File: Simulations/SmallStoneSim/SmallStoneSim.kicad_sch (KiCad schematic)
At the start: 77 parts, among them Q1 2N5088, Q2 2N5087, Q3 2N5088, Q4 2N5087, Q5 2N5087, Q6 2N5088, Q7 2N5088, SW1 SW_SPDT, SW2 SW_SPDT, U1 LM13700, U2 LM13700, U3 LM13700

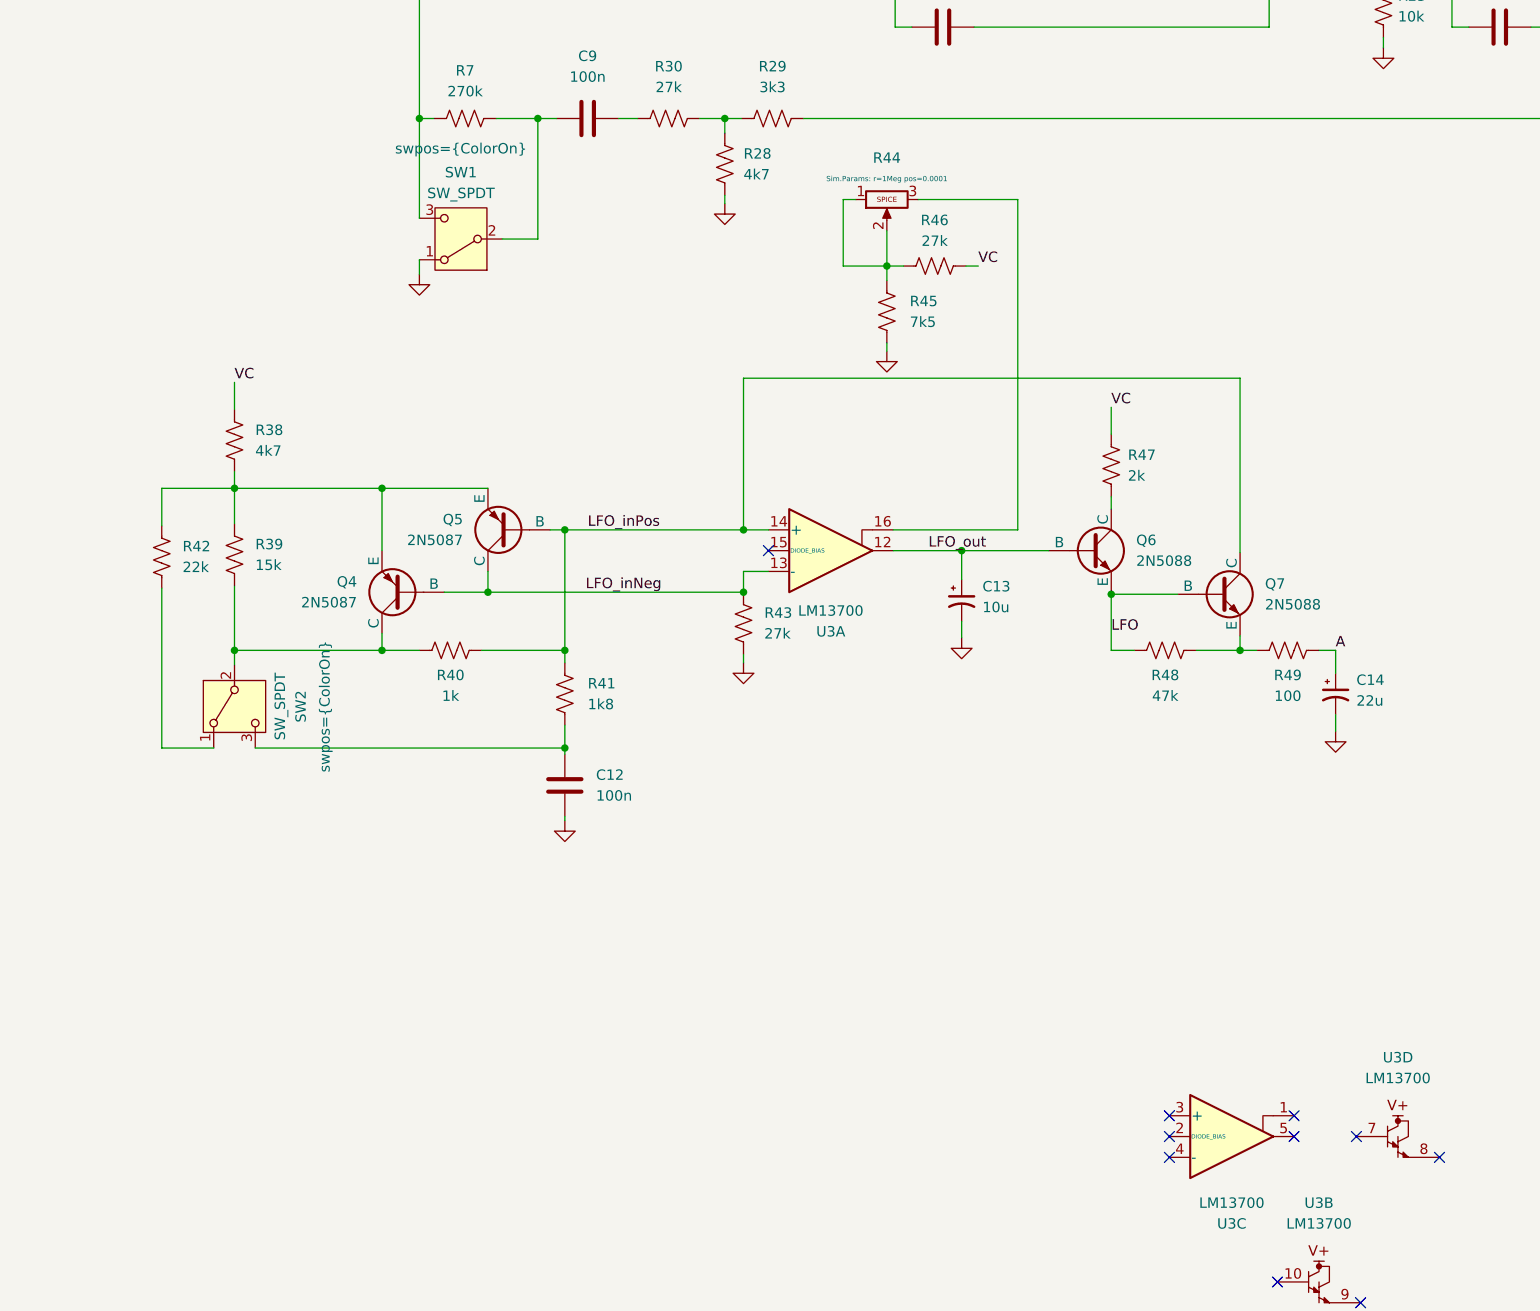
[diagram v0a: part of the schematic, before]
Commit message: New circuit sim
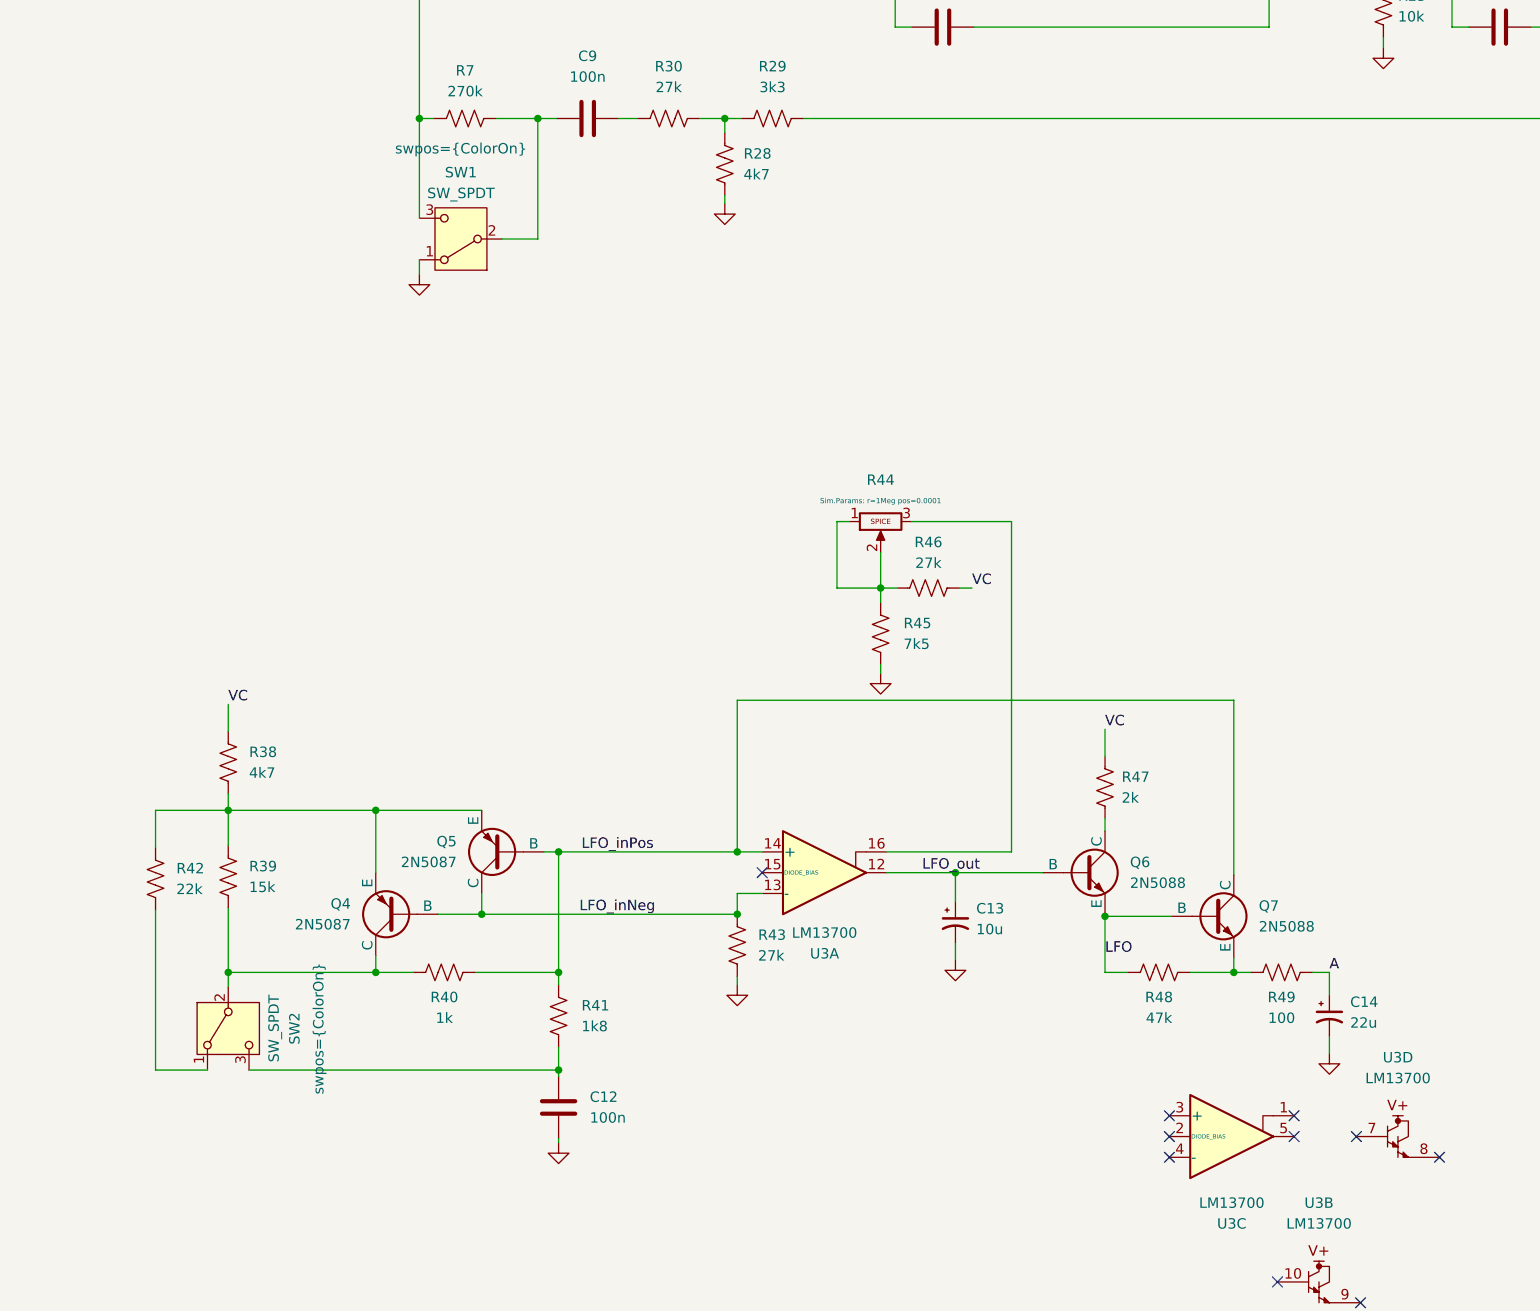
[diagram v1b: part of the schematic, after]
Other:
- moved on the sheet: C12, C13, C14, Q4, Q5, Q6, Q7, R38, R39, R40, R41, R42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
